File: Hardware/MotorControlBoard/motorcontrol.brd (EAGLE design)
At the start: 52.5 x 39 mm, 27 parts, among them U1 ATMEGA328P-AU

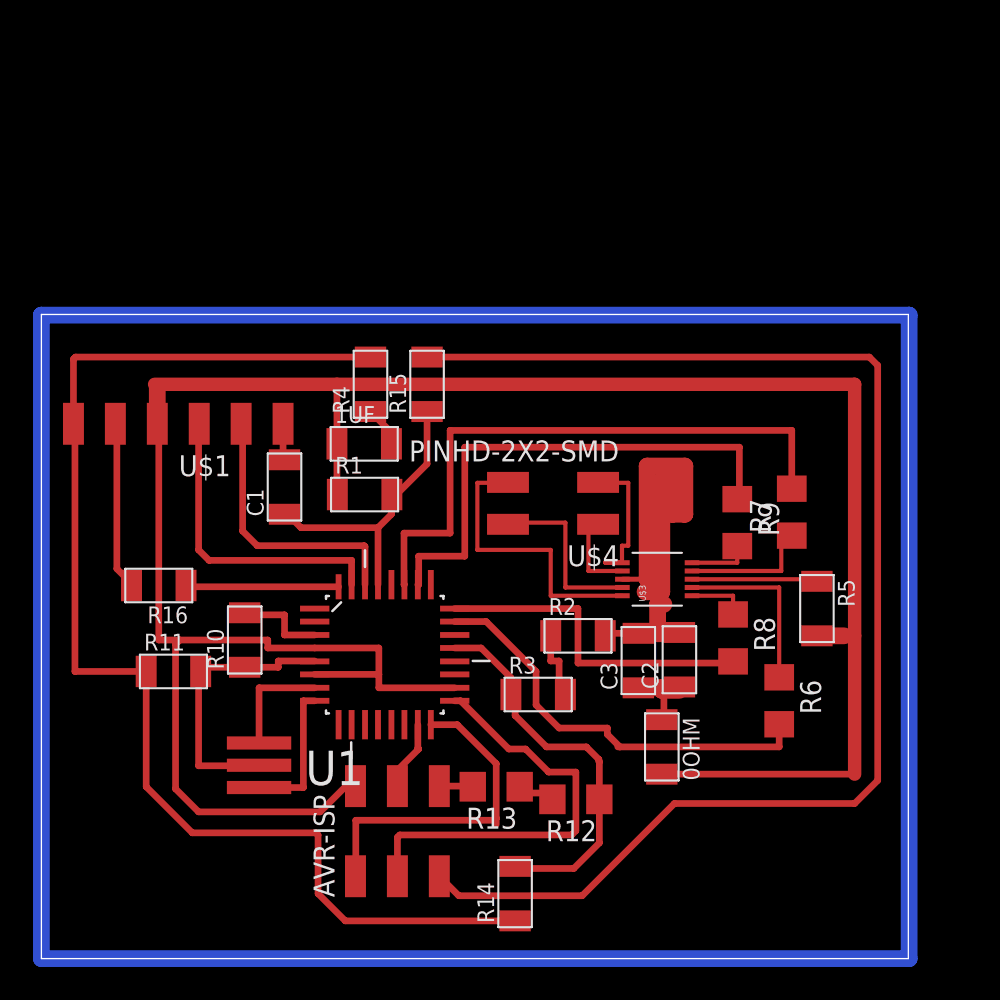
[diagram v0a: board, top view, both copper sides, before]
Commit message: new board
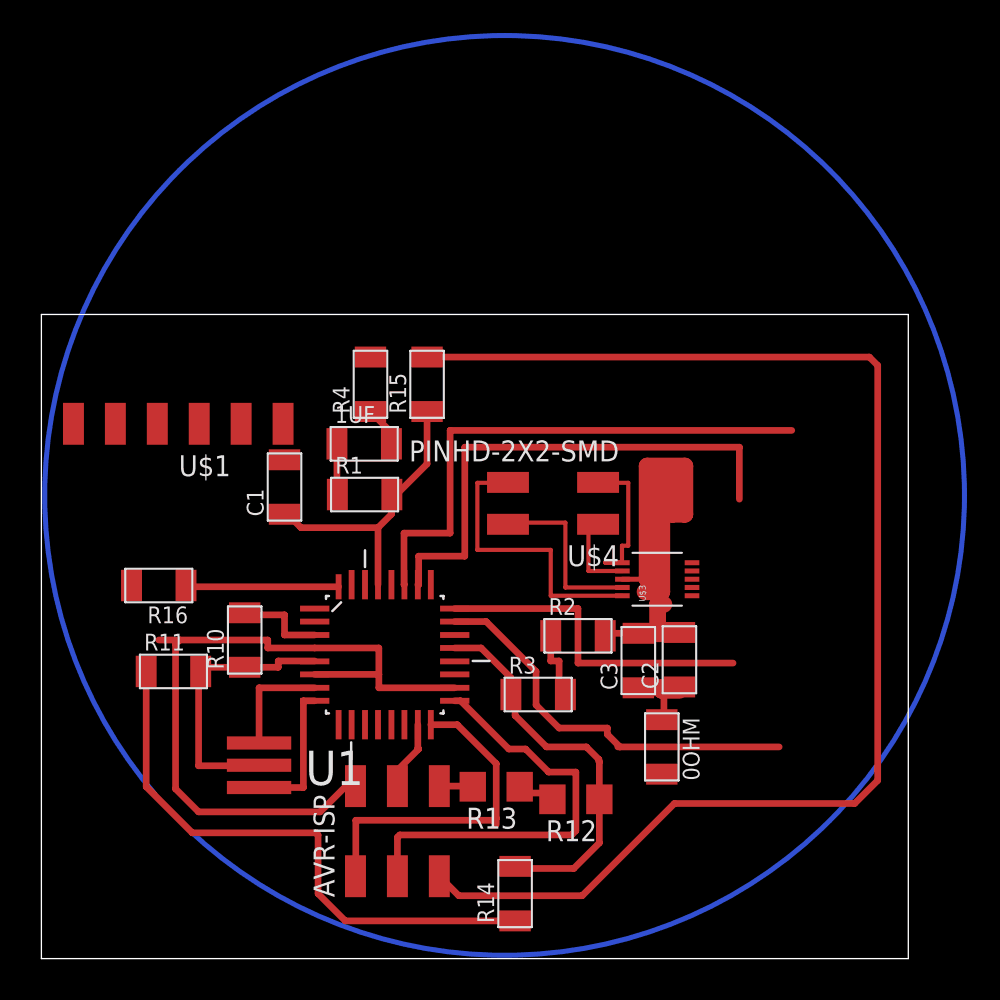
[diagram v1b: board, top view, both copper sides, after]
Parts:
- removed R5: 0, fab:R1206FAB
- removed R6, R7, R8, R9: 0, fab:R1206
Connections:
- removed net N$1: R5.1, U$3.3
- removed net N$2: R6.1, U$3.2
- removed net N$3: R7.1, U$3.4
- removed net N$4: R8.1, U$3.1
- removed net N$5: R9.2, U$3.5
- net IN1A: now also U$3.2; no longer R6.2
- net IN1B: now also U$3.4; no longer R7.2
- net IN2A: now also U$3.1; no longer R8.2
- net IN2B: now also U$3.5; no longer R9.1
- net VCC: now also U$3.3; no longer R5.2
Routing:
- net N$9: track 183.1 -> 0.00 mm
- net VCC: track 148.3 -> 49.5 mm
- net GND: track 76.5 -> 35.2 mm
- net TX: track 18.6 -> 0.00 mm
- net RX: track 16.5 -> 0.00 mm
- net N$2: track 10.7 -> 0.00 mm
- net N$7: track 10.2 -> 0.00 mm
- net N$3: track 8.24 -> 0.00 mm
- net N$1: track 7.69 -> 0.00 mm
- net N$5: track 3.75 -> 0.00 mm
- net N$4: track 3.62 -> 0.00 mm
- net IN1B: track 36.4 -> 32.9 mm
- net N$10: track 2.21 -> 0.00 mm
- net IN1A: track 25.7 -> 24.3 mm
